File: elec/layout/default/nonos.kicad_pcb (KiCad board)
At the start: 2 copper layers, 45 x 122 mm, 62 parts, among them CN1 HRSHirose_DF40C_100DS_0_4V51, CN2 HRSHirose_DF40C_100DS_0_4V51, Q1 MOSFET, U1 STUSB4500QTR, U2 _Texas_Instruments_SN74LVC1G0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, U3 _Texas_Instruments_TAS5825MRH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, U4 Texas_Instruments_TPS56637RPAR, U5 JST_Sales_America_B02B_XASK_1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, U6 JST_Sales_America_B02B_XASK_1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

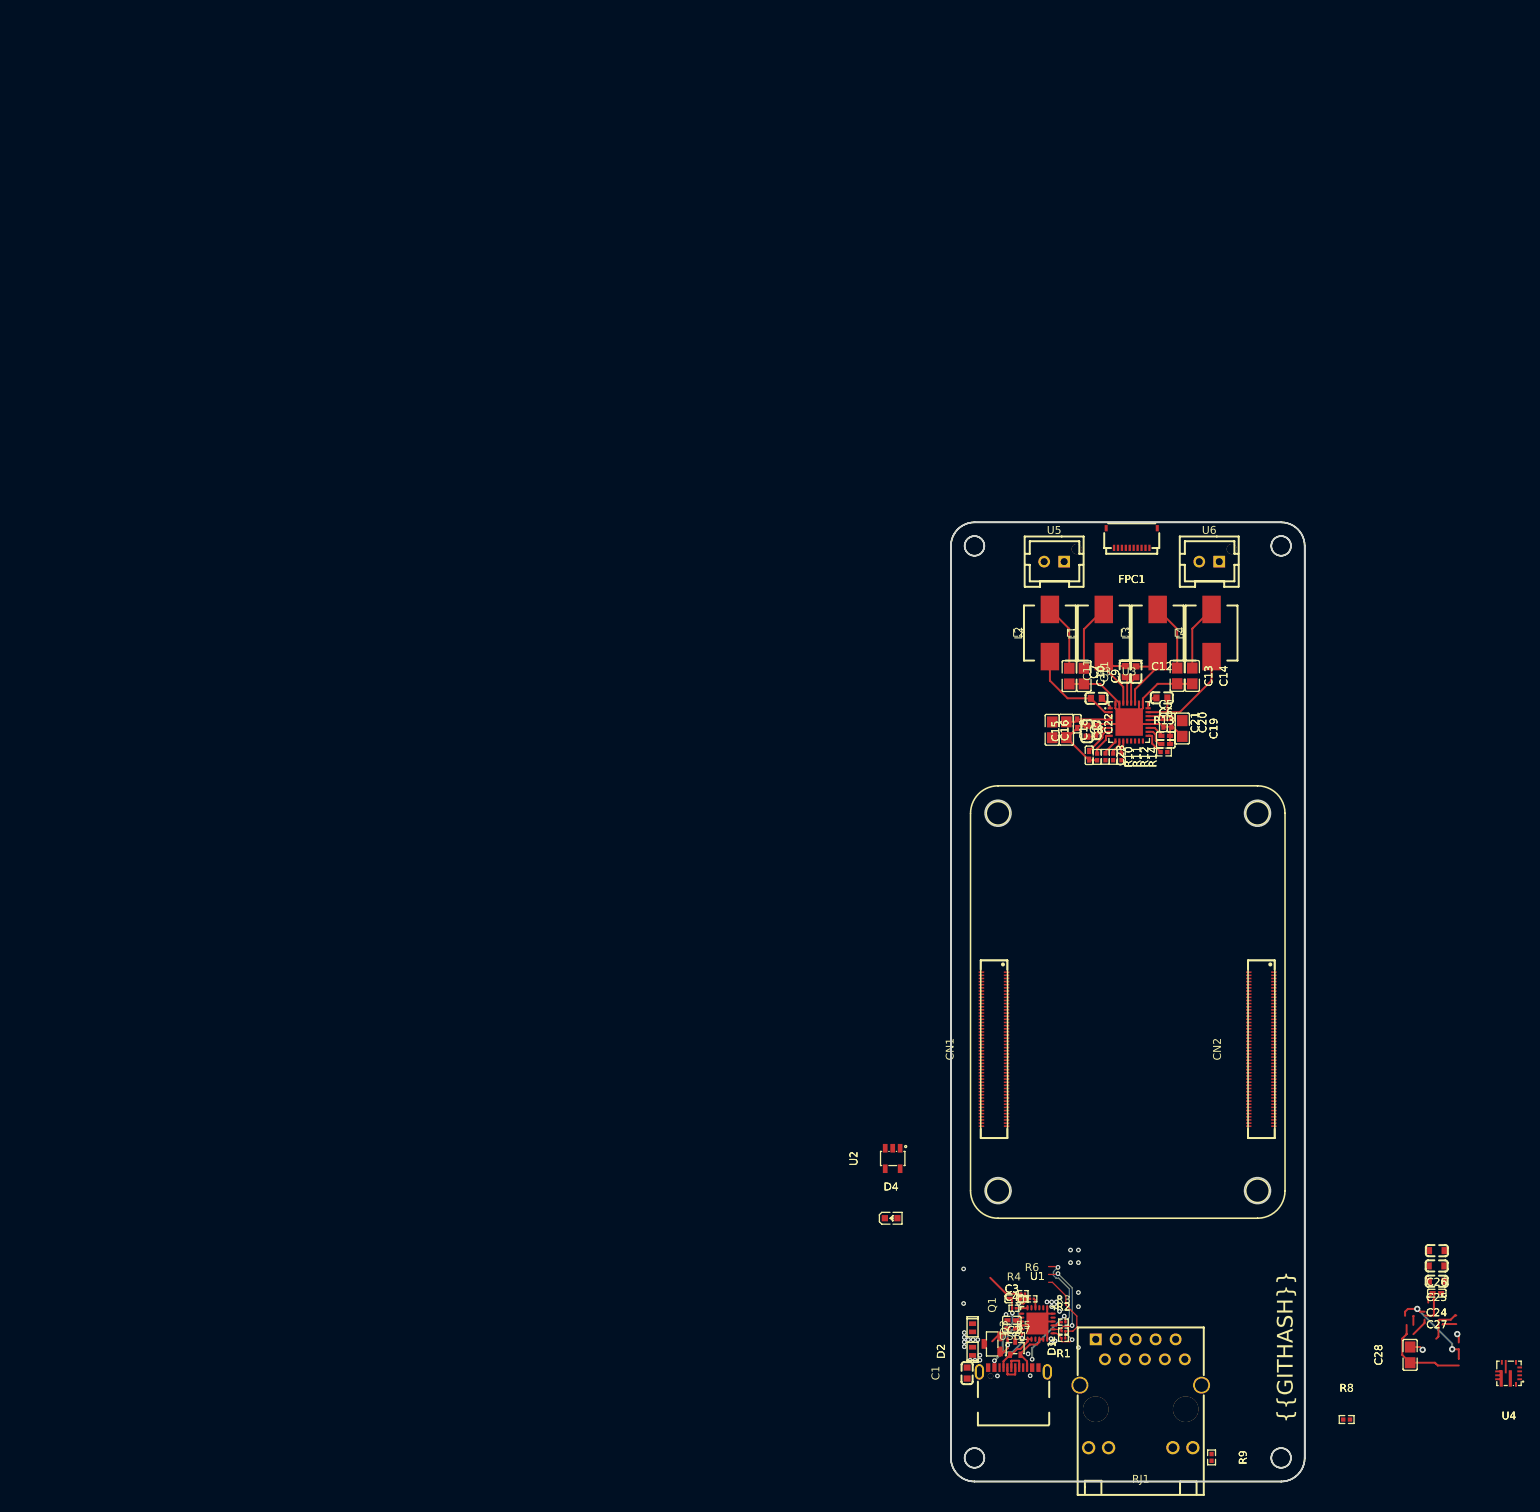
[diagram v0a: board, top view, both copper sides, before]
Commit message: builds working
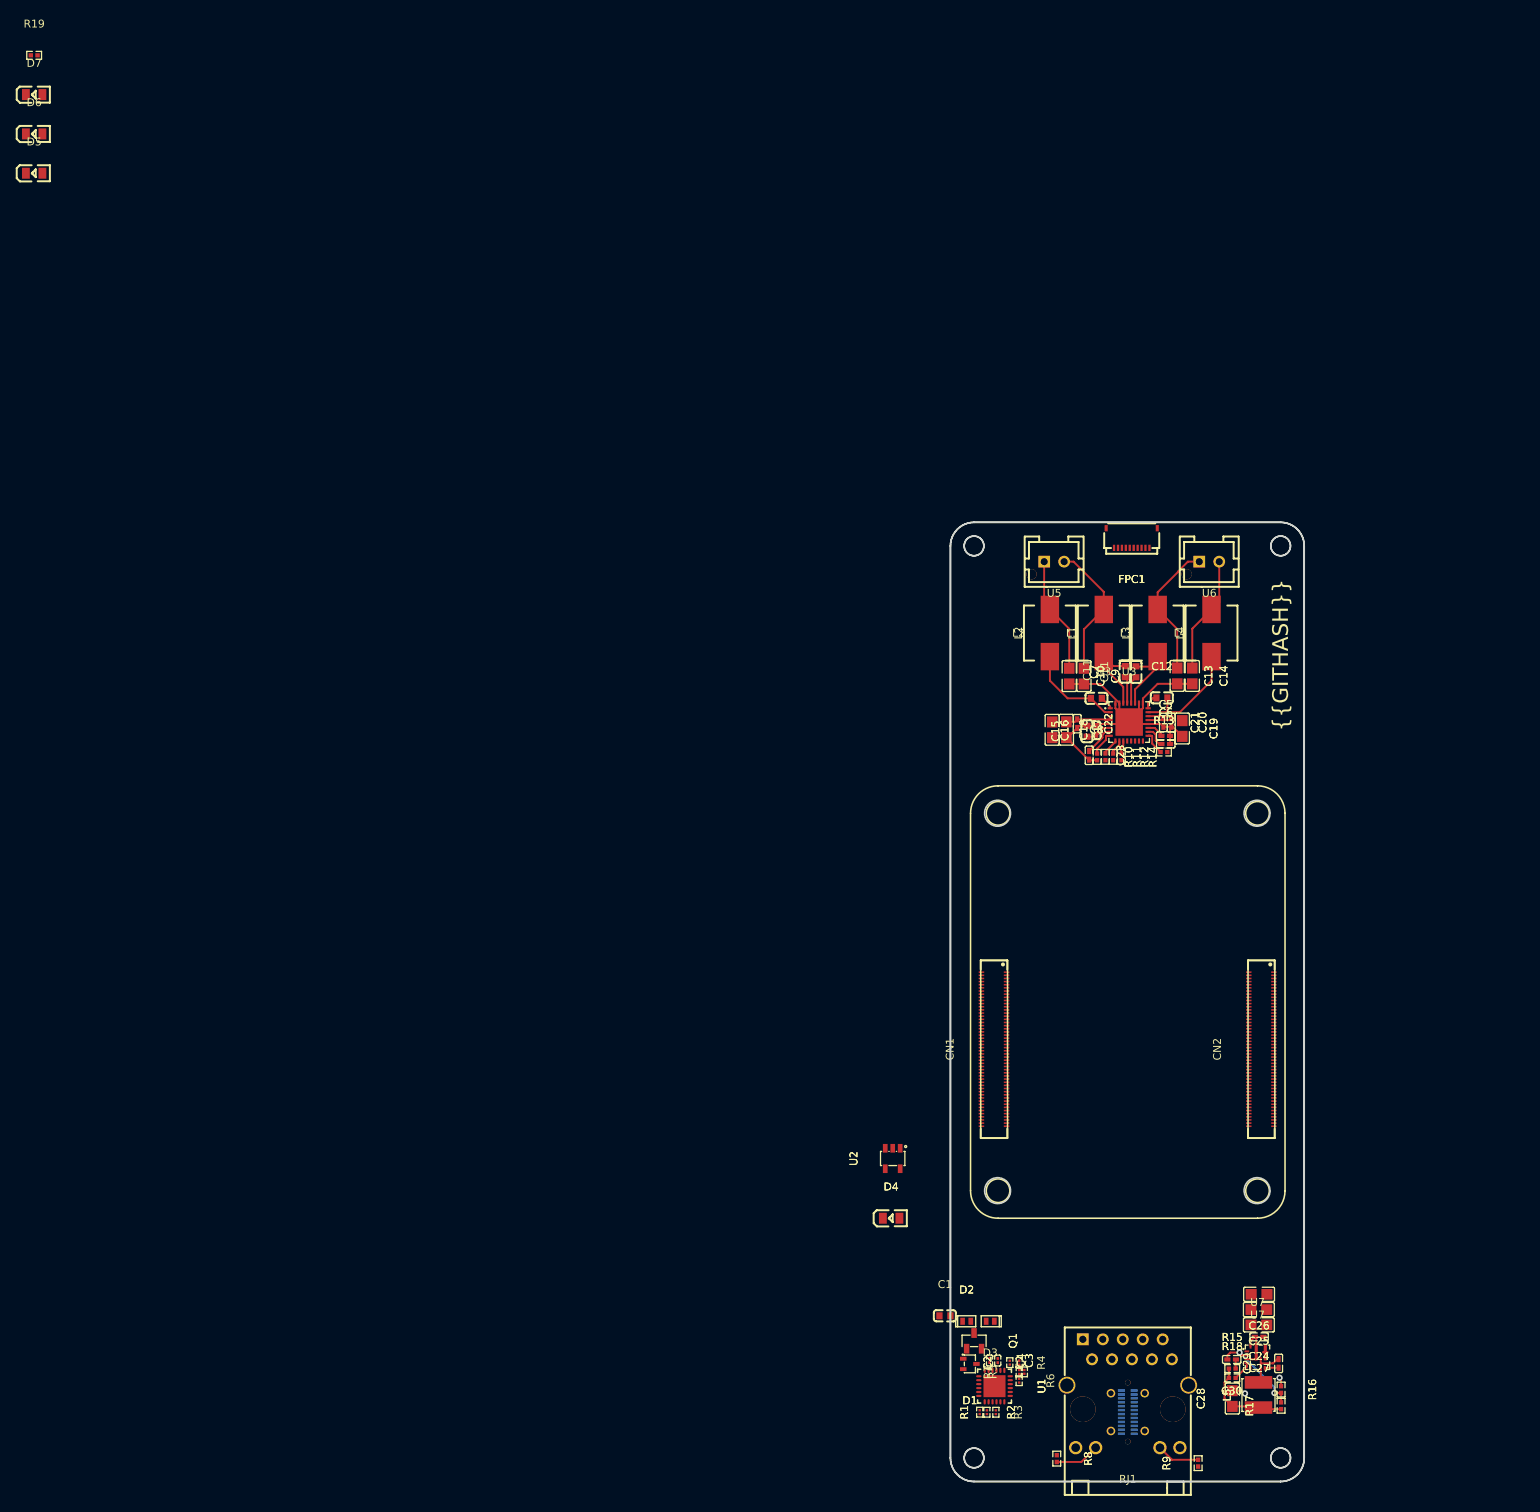
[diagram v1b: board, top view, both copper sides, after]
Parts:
- removed USB1: TYPE_C_16PIN_2MD073, lcsc:USB-C-SMD_TYPE-C-6PIN-2MD-073
- added C29: 100nF ±10% 16V X7R, lcsc:C0402, F.Cu at (158.3, 151.4)
- added C30: 100pF ±5% 50V C0G, lcsc:C0402, F.Cu at (152.3, 150.9)
- added D5: , lcsc:LED0805-R-RD, F.Cu at (0.00, 0.00)
- added D6: , lcsc:LED0805-R-RD, F.Cu at (0.00, -5.00)
- added D7: , lcsc:LED0805-R-RD, F.Cu at (0.00, -10.0)
- added L5: 3.3µH ±20% 4A 73mΩ, lcsc:IND-SMD_L4.0-W4.0, F.Cu at (155.7, 155.4)
- added R15: 22kΩ ±1% 62.5mW, lcsc:R0402, F.Cu at (152.4, 152.0)
- added R16: 8.2kΩ ±1% 62.5mW, lcsc:R0402, F.Cu at (158.6, 154.7)
- added R17: 68kΩ ±1% 62.5mW, lcsc:R0402, F.Cu at (158.6, 156.8)
- added R18: 100kΩ ±1% 62.5mW, lcsc:R0402, F.Cu at (152.4, 153.2)
- added R19: 5.1kΩ ±1% 62.5mW, lcsc:R0402, F.Cu at (0.00, -15.0)
- added U7: _Texas_Instruments_TPS56637RPAR, lcsc:VQFN-HR-10_L3.0-W3.0_RPA, F.Cu at (155.6, 150.6)
- C10, C13, C14: value (none) -> 680nF ±10% 50V X7R
- C11, C12, C8: value (none) -> 470nF ±10% 50V X7R
- C18, C19: value (none) -> 22µF ±20% 25V X5R
- C2: value (none) -> 100nF ±10% 10V X5R; footprint lcsc:C0402 -> lcsc:C0201
- C20, C21, C22, C27: value (none) -> 100nF ±10% 16V X7R
- C23, C5: value (none) -> 1µF ±10% 25V X5R
- C24, C25, C26: value (none) -> 4.7µF ±10% 25V X5R; footprint lcsc:C0603 -> lcsc:C0805
- C3, C4: value (none) -> 1µF ±20% 6.3V X5R; footprint lcsc:C0402 -> lcsc:C0201
- D4: value 2.7V -> (none); footprint lcsc:LED0603-RD_WHITE -> lcsc:LED0805-R-RD
- L1, L3, L4: value (none) -> 10µH ±20% 4.5A 68mΩ
- Q1: footprint lcsc:SOT-23-3_L2.9-W1.3-P1.90-LS2.4-BR -> lcsc:SOT-23-3_L2.9-W1.3-P1.90-LS2.4-BR-1
- R1: value (none) -> 1kΩ ±1% 50mW
- R12, R13, R14: value (none) -> 10kΩ ±1% 62.5mW
- R2: value 4.64kΩ ±1% 50mW -> 4.7kΩ ±1% 50mW
- R3: value (none) -> 4.7kΩ ±1% 50mW
- R8: value 453Ω ±1% 62.5mW -> 470Ω ±1% 62.5mW
- R9: value (none) -> 470Ω ±1% 62.5mW
- U4: value Texas_Instruments_TPS56637RPAR -> _HCTL_HC_TYPE_C_24P_VS9_3_5A_F1_1_04; footprint lcsc:VQFN-HR-10_L3.0-W3.0_RPA -> lcsc:USB-C-SMD_HC-TYPE-C-24P-VS9.3-5A-F1.1-04; moved to B.Cu
- moved U4 48.7 mm to (139.1, 157.6), turned to -90 degrees
- moved R8 37.2 mm to (130.1, 163.5), turned to -90 degrees
- moved C25 23.3 mm to (155.8, 144.5)
- moved C26 23.3 mm to (155.8, 142.6)
- moved C27 23.3 mm to (155.8, 148.0)
- moved C24 23.3 mm to (155.8, 146.5)
- moved C28 23.3 mm to (152.4, 155.8)
- moved R1 14.3 mm to (122.3, 157.6), turned to 90 degrees
- moved R2 14.2 mm to (120.3, 157.6), turned to -90 degrees
- moved R3 14.2 mm to (121.2, 157.6), turned to -90 degrees
- moved R6 10.5 mm to (125.3, 153.6), turned to -90 degrees
- moved R5 9.95 mm to (125.9, 152.5), turned to 90 degrees
- moved U1 9.65 mm to (122.1, 154.3), turned to -90 degrees
- moved R7 9.33 mm to (125.3, 152.5), turned to 90 degrees
- moved C2 8.17 mm to (125.3, 151.3), turned to 90 degrees
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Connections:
- net pins[47] renamed processor-signal-7
- net processor-pins[40] renamed processor-signal-8
- net processor.hdi_b-pins[40] renamed pins[40]
- C10 pad 1: net-1 -> net
- C10 pad 2: amplifier-net-6 -> lv
- C11 pad 1: amplifier-net-4 -> amplifier-net-6
- C11 pad 2: amplifier-net-12 -> amplifier-net-4
- C12 pad 1: amplifier-net-1 -> amplifier-net-5
- C12 pad 2: amplifier-net-2 -> amplifier-net-3
- C13 pad 1: net-3 -> net-4
- C13 pad 2: amplifier-net-6 -> lv
- C14 pad 2: amplifier-net-6 -> lv
- C15 pad 1: DVDD -> VCC_3V3
- C15 pad 2: amplifier-net-6 -> lv
- C16 pad 1: DVDD -> VCC_3V3
- C16 pad 2: amplifier-net-6 -> lv
- C17 pad 1: PVDD -> VSINK_VCC
- C17 pad 2: amplifier-net-6 -> lv
- C18 pad 1: PVDD -> VSINK_VCC
- C18 pad 2: amplifier-net-6 -> lv
- C19 pad 1: PVDD -> VSINK_VCC
- C19 pad 2: amplifier-net-6 -> lv
- C2 pad 1: pd_controller-net -> pd_controller-net-2
- C20 pad 1: PVDD -> VSINK_VCC
- C20 pad 2: amplifier-net-6 -> lv
- C21 pad 1: PVDD -> VSINK_VCC
- C21 pad 2: amplifier-net-6 -> lv
- C22 pad 1: PVDD -> VSINK_VCC
- C22 pad 2: amplifier-net-6 -> lv
- C23 pad 2: amplifier-net-6 -> lv
- C28 pad 1: hv -> net-3
- C5 pad 2: amplifier-net-6 -> lv
- C6 pad 1: amplifier-net-11 -> amplifier-net-9
- C6 pad 2: amplifier-net-6 -> lv
- C7 pad 1: amplifier-net-5 -> amplifier-net-10
- C7 pad 2: amplifier-net -> amplifier-net-2
- C8 pad 1: amplifier-net-10 -> amplifier-net
- C8 pad 2: amplifier-net-3 -> amplifier-net-1
- C9 pad 1: net -> net-1
- C9 pad 2: amplifier-net-6 -> lv
- CN1 pad 15: signal-6 -> signal-1
- CN1 pad 17: signal-7 -> signal-3
- CN1 pad 19: processor-signal-1 -> processor-signal-5
- CN1 pad 23: processor-signal-5 -> processor-signal
- CN1 pad 28: signal-3 -> signal-5
- CN1 pad 29: signal-1 -> signal-6
- CN1 pad 73: pins[54] -> processor-signal-1
- CN1 pad 77: processor-pins[46]-1 -> processor-pins[46]
- CN1 pad 78: processor-signal -> processor-signal-4
- CN1 pad 82: signal-5 -> signal-2
- CN1 pad 85: processor-signal-2 -> pins[30]
- CN1 pad 86: processor-signal-4 -> processor-signal-6
- CN1 pad 87: processor-signal-6 -> processor-signal-2
- CN2 pad 77: processor-pins[46] -> processor-pins[46]-1
- D4 pad 1: net-4 -> processor-net
- D4 pad 2: VCC_3V3 -> processor-net-1
- FPC1 pad 10: signal-5 -> signal-2
- FPC1 pad 4: hv -> net-3
- FPC1 pad 6: lv-1 -> lv
- FPC1 pad 8: signal-7 -> signal-3
- FPC1 pad 9: signal-6 -> signal-1
- L1 pad 1: amplifier-net -> amplifier-net-2
- L1 pad 2: net -> net-1
- L2 pad 1: amplifier-net-3 -> amplifier-net-1
- L2 pad 2: net-1 -> net
- L3 pad 1: amplifier-net-12 -> amplifier-net-4
- L3 pad 2: net-3 -> net-4
- L4 pad 1: amplifier-net-2 -> amplifier-net-3
- Q1 pad 1: pd_controller-net-1 -> pd_controller-net
- R10 pad 1: amplifier-net-9 -> amplifier-net-11
- R10 pad 2: amplifier-net-6 -> lv
- R11 pad 1: signal-1 -> signal-6
- R12 pad 1: signal -> signal-7
- R13 pad 1: signal-3 -> signal-5
- R14 pad 1: signal-2 -> signal
- R2 pad 2: pd_controller-hv -> hv
- R3 pad 2: pd_controller-hv -> hv
- R4 pad 2: pd_controller-net-2 -> pd_controller-net-1
- R5 pad 1: pd_controller-net-1 -> pd_controller-net
- R6 pad 1: pd_controller-net-1 -> pd_controller-net
- R7 pad 1: pd_controller-net-1 -> pd_controller-net
- R7 pad 2: pd_controller-net -> pd_controller-net-2
- RJ1 pad SHIELD0: lv-1 -> lv
- RJ1 pad SHIELD1: lv-1 -> lv
- U1 pad 18: pd_controller-net-2 -> pd_controller-net-1
- U2 pad 4: net-4 -> processor-net
- U3 pad 1: amplifier-net-10 -> amplifier-net
- U3 pad 10: signal -> signal-7
- U3 pad 11: signal-2 -> signal
- U3 pad 17: signal-3 -> signal-5
- U3 pad 18: amplifier-net-11 -> amplifier-net-9
- U3 pad 2: amplifier-net-3 -> amplifier-net-1
- U3 pad 20: amplifier-net-6 -> lv
- U3 pad 21: PVDD -> VSINK_VCC
- U3 pad 22: PVDD -> VSINK_VCC
- U3 pad 23: amplifier-net-2 -> amplifier-net-3
- U3 pad 24: amplifier-net-1 -> amplifier-net-5
- U3 pad 25: amplifier-net-6 -> lv
- U3 pad 26: amplifier-net-6 -> lv
- U3 pad 27: amplifier-net-12 -> amplifier-net-4
- U3 pad 28: amplifier-net-4 -> amplifier-net-6
- U3 pad 29: amplifier-net-5 -> amplifier-net-10
- U3 pad 3: PVDD -> VSINK_VCC
- U3 pad 30: amplifier-net -> amplifier-net-2
- U3 pad 31: amplifier-net-6 -> lv
- U3 pad 32: amplifier-net-6 -> lv
- U3 pad 33: amplifier-net-6 -> lv
- U3 pad 4: PVDD -> VSINK_VCC
- U3 pad 5: amplifier-net-6 -> lv
- U3 pad 6: DVDD -> VCC_3V3
- U3 pad 8: amplifier-net-9 -> amplifier-net-11
- U3 pad 9: signal-1 -> signal-6
- U5 pad 1: net-1 -> net
- U5 pad 2: net -> net-1
- U6 pad 1: net-2 -> net-4
- U6 pad 2: net-3 -> net-2
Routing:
- net amplifier-net-6: track 50.8 -> 1.70 mm
- net lv: track 20.0 -> 59.2 mm
- net VBUS: track 24.6 -> 0.00 mm, vias 11 -> 0
- net net-4: track 0.00 -> 17.4 mm
- net I2C_SCL: track 15.2 -> 0.00 mm, vias 2 -> 0
- net PVDD: track 14.5 -> 0.00 mm
- net regulator-net-3: track 0.00 -> 12.3 mm, vias 0 -> 2
- net I2S_WS: track 12.3 -> 0.00 mm, vias 2 -> 0
- net pd_controller-net-1: track 12.1 -> 0.00 mm, vias 2 -> 0
- net hv: track 11.8 -> 0.00 mm
- net I2C_SDA: track 11.6 -> 0.00 mm, vias 2 -> 0
- net amplifier-net-5: track 3.41 -> 14.6 mm
- net amplifier-net-12: track 10.8 -> 0.00 mm
- net amplifier-net-7: track 2.20 -> 12.4 mm
- net pd_controller-hv: track 10.1 -> 0.00 mm
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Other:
- board text removed: "USBPD DEV BOARD"
